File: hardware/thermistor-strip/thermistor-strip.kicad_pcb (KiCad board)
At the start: 2 copper layers, 158 x 13.5 mm, 7 parts, among them J1 FH19C-7S-0.5SH10

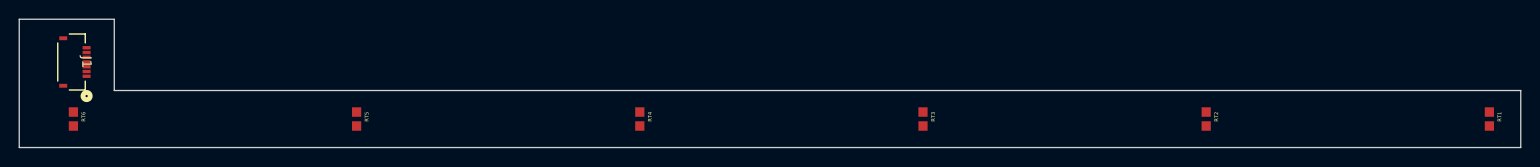
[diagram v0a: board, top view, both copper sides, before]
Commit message: initial tracing progress
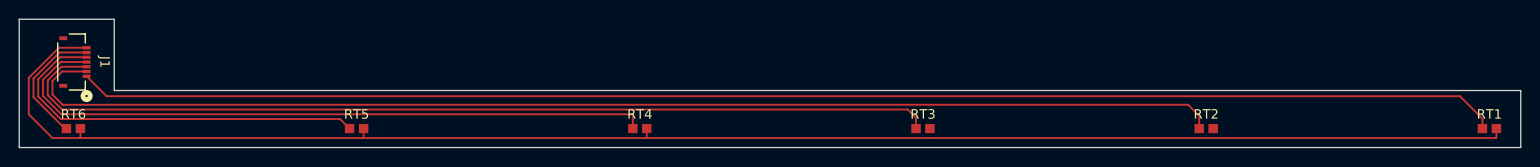
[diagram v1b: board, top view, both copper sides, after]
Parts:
- moved RT1 1.00 mm to (204.7, 148.0), turned to 0 degrees
- moved RT2 1.00 mm to (174.9, 148.0), turned to 0 degrees
- moved RT3 1.00 mm to (145.1, 148.0), turned to 0 degrees
- moved RT4 1.00 mm to (115.3, 148.0), turned to 0 degrees
- moved RT5 1.00 mm to (85.5, 148.0), turned to 0 degrees
- moved RT6 1.00 mm to (55.7, 148.0), turned to 0 degrees
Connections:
- J1 pad 1: GND -> Net-(J1-Pad1)
- J1 pad 7: Net-(J1-Pad7) -> GND
- RT1 pad 1: Net-(J1-Pad7) -> Net-(J1-Pad1)
- RT2 pad 1: Net-(J1-Pad6) -> Net-(J1-Pad2)
- RT3 pad 1: Net-(J1-Pad5) -> Net-(J1-Pad3)
- RT5 pad 1: Net-(J1-Pad3) -> Net-(J1-Pad5)
- RT6 pad 1: Net-(J1-Pad2) -> Net-(J1-Pad6)
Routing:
- net GND: track 0.00 -> 170.7 mm
- net Net-(J1-Pad1): track 0.00 -> 149.8 mm
- net Net-(J1-Pad2): track 0.00 -> 128.4 mm
- net Net-(J1-Pad3): track 0.00 -> 99.7 mm
- net Net-(J1-Pad4): track 0.00 -> 71.4 mm
- net Net-(J1-Pad5): track 0.00 -> 42.0 mm
- net Net-(J1-Pad6): track 0.00 -> 13.5 mm
